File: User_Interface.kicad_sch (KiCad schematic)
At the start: 5 parts, among them Q4 MMBT2222A, SW2 Estop, SW3 SW_Push

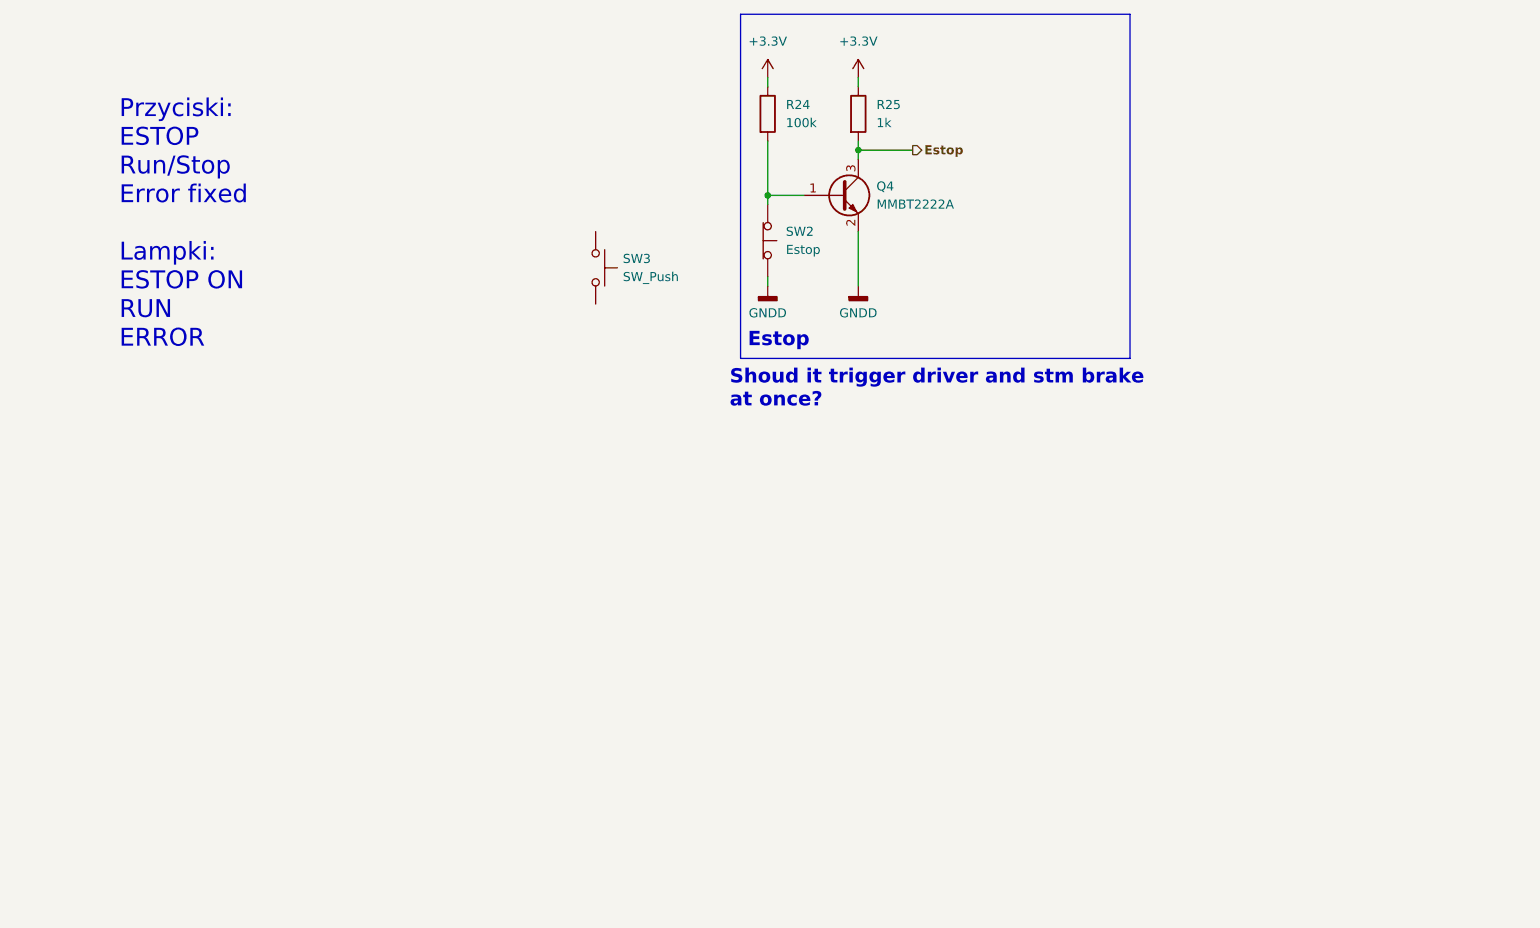
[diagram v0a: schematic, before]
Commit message: 90% schematic first layout
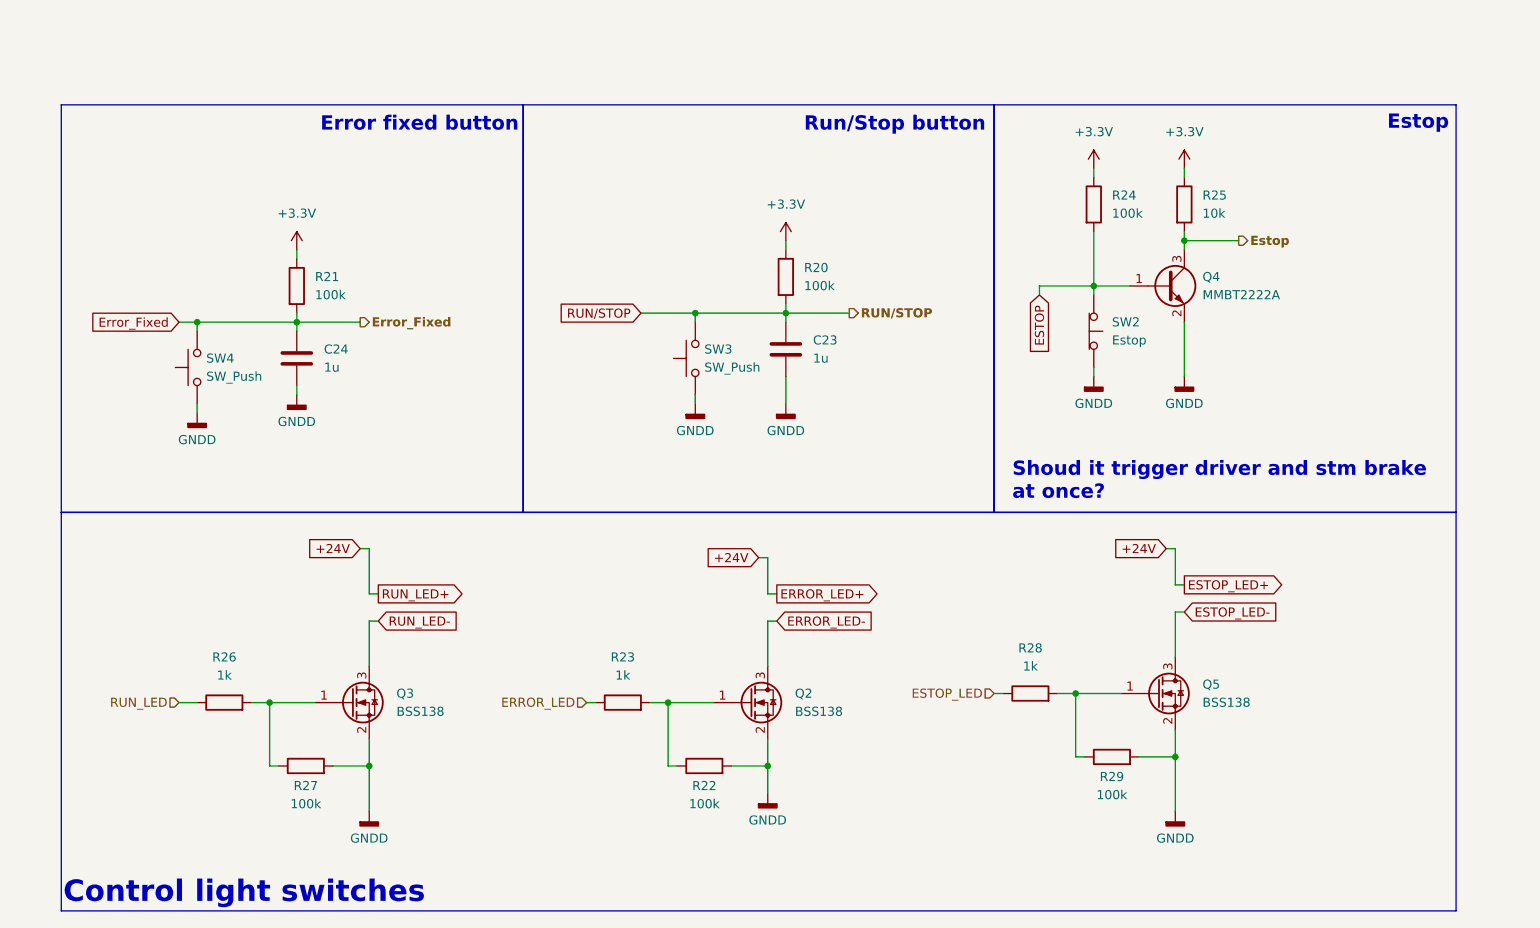
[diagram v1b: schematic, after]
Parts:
- added C23, C24: 1u, Capacitor_SMD:C_0805_2012Metric_Pad1.18x1.45mm_HandSolder, symbol Device:C
- added Q2, Q3, Q5: BSS138, Package_TO_SOT_SMD:SOT-23, symbol Transistor_FET:BSS138
- added R20, R21, R22, R27, R29: 100k, Resistor_SMD:R_0805_2012Metric, symbol Device:R
- added R23, R26, R28: 1k, Resistor_SMD:R_0805_2012Metric, symbol Device:R
- added SW4: SW_Push, Button_Switch_THT:SW_PUSH_6mm_H5mm, symbol Switch:SW_Push
- R25: value 1k -> 10k
- SW3: footprint (none) -> Button_Switch_THT:SW_PUSH_6mm_H5mm
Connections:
- net +3.3V: now also R20.1, R21.1
- net GNDD: now also SW3.1, C23.2, C24.2, Q2.2 (S), Q3.2 (S), Q5.2 (S), R22.2, R27.2, R29.2, SW4.1
- net ESTOP: now reaches Q4.1 (B), R24.2, SW2.1 (A)
- net RUN/STOP: now reaches SW3.2
- net RUN/STOP: now also C23.1, R20.2
- new net: Q3.1 (G), R26.2, R27.1
- new net: Q5.1 (G), R28.2, R29.1
- new net: Q2.1 (G), R22.1, R23.2
- new net ERROR_LED: R23.1
- new net ERROR_LED-: Q2.3 (D)
- new net ESTOP_LED: R28.1
- new net ESTOP_LED-: Q5.3 (D)
- new net Error_Fixed: C24.1, R21.2, SW4.2
- new net RUN_LED: R26.1
- new net RUN_LED-: Q3.3 (D)
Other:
- note added: "Control light switches"
- note added: "Error fixed button"
- note added: "Run/Stop button"
- note removed: "Przyciski: ESTOP Run/Stop Error fixed Lampki: ESTOP ON RUN ERROR"
- moved on the sheet: Q4, R24, R25, SW2
